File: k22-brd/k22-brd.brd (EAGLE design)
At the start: 22.9 x 63.5 mm, 34 parts, among them J1 61302011121, J2 61302011121, J3 CORTEX_DEBUG_PTH

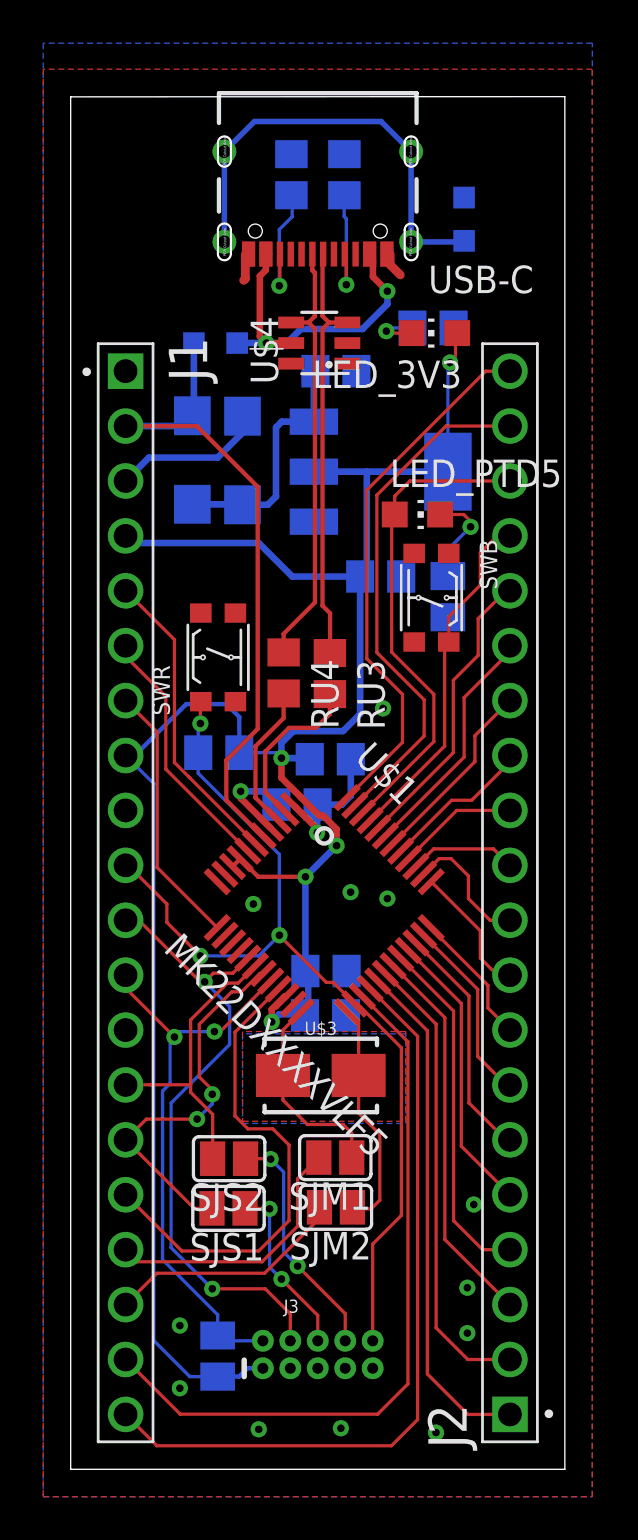
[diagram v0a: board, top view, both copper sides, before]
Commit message: prezehleno
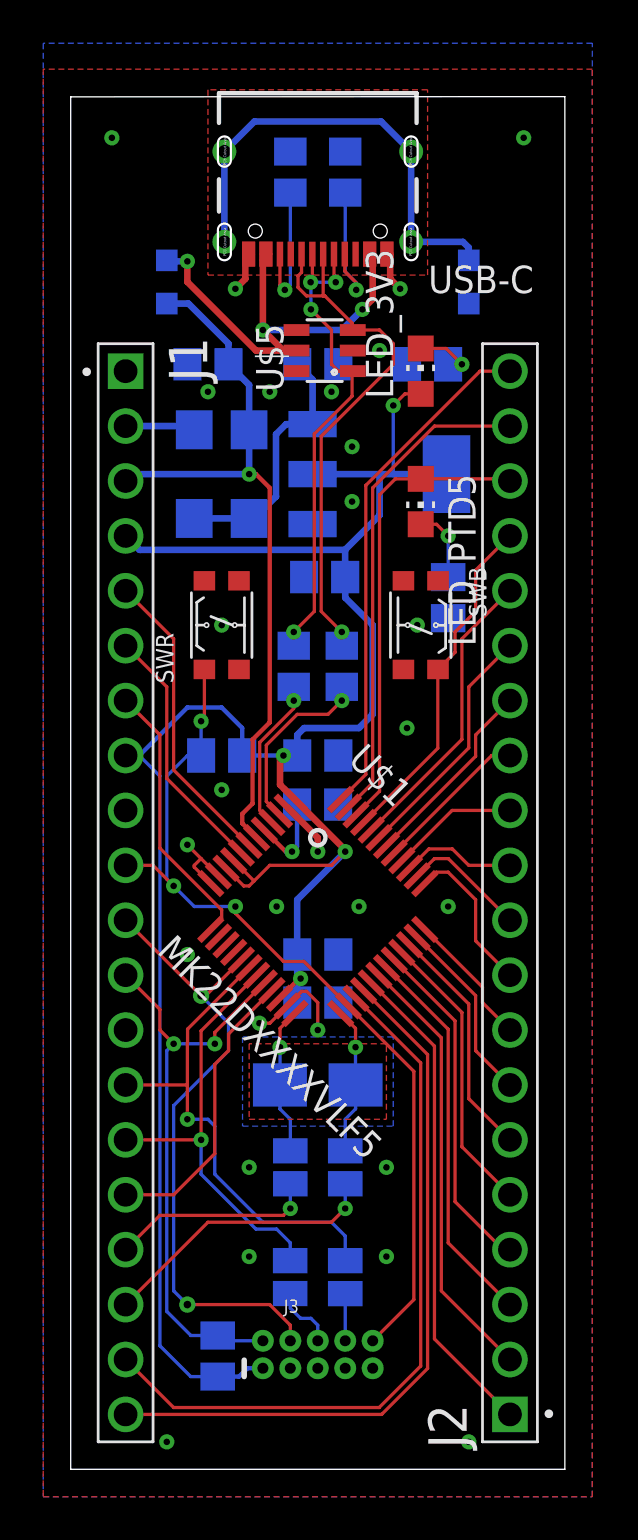
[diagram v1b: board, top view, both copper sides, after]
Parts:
- removed U$4: USBLC6-4SC6Y, vym0038_k22_misc:SOT23-6L
- added CU1: <1,10>u, rcl:C0805
- added U$5: USBLC6-2SC6, vym0038_k22_misc:SOT23-6L
- moved SJS2 7.67 mm to (12.7, 8.89), flipped to the bottom, turned to 90 degrees
- moved SJS1 4.27 mm to (10.2, 8.89), flipped to the bottom, turned to 90 degrees
- moved LU1 3.62 mm to (4.45, 54.9), turned to 90 degrees
- moved LU2 2.91 mm to (18.4, 54.9), turned to 90 degrees
- moved DV1 2.70 mm to (8.26, 46.0)
- moved CV2 2.59 mm to (11.7, 41.3), turned to 0 degrees
- moved DV2 2.32 mm to (5.71, 46.0)
- moved SJM1 2.13 mm to (10.2, 14.0), flipped to the bottom, turned to 270 degrees
- moved SJM2 1.90 mm to (12.7, 14.0), flipped to the bottom, turned to 270 degrees
- moved LED_3V3 1.87 mm to (16.2, 50.8), turned to 0 degrees
- moved RV1 1.70 mm to (16.5, 51.1), turned to 0 degrees
- moved SWR 1.50 mm to (6.99, 39.1)
- moved SWB 1.36 mm to (16.2, 39.1)
- moved CM4 0.95 mm to (11.4, 30.8)
- moved CV1 0.90 mm to (11.4, 51.1)
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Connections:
- net D+CON: now also U$5.3, U$5.4; no longer U$4.3
- net D-CON: now also U$5.1, U$5.6; no longer U$4.4
- net GND: now also CU1.1, U$5.2; no longer U$4.2
- net USB5V: now also CU1.2, J1.3; no longer J1.2
- net VBUSCON: now also U$5.5; no longer U$4.5
- net VIN: now also J1.2; no longer J1.3
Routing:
- net UART_RX: track 13.9 -> 23.0 mm, vias 0 -> 1
- net PTA4: track 22.5 -> 13.6 mm
- net N$3: track 11.0 -> 2.18 mm, vias 2 -> 0
- net GND: track 8.83 -> 15.3 mm, vias 13 -> 28
- net VBUSCON: track 16.6 -> 22.2 mm, vias 2 -> 3
- net N$4: track 8.17 -> 2.99 mm, vias 2 -> 0
- net D+CON: track 20.0 -> 24.9 mm, vias 0 -> 1
- net PTA19_OSC: track 10.8 -> 6.84 mm, vias 0 -> 1
- net VIN: track 7.10 -> 3.25 mm
- net PTA18: track 12.5 -> 9.55 mm, vias 0 -> 1
- net D-CON: track 20.1 -> 23.0 mm, vias 0 -> 4
- net PTA18_OSC: track 9.39 -> 6.84 mm, vias 0 -> 1
- net USB5V: track 31.6 -> 34.1 mm, vias 0 -> 1
- net UART_TX: track 17.9 -> 20.0 mm, vias 2 -> 1
- net RESET: track 44.1 -> 42.0 mm
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
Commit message: Nejake zmeny
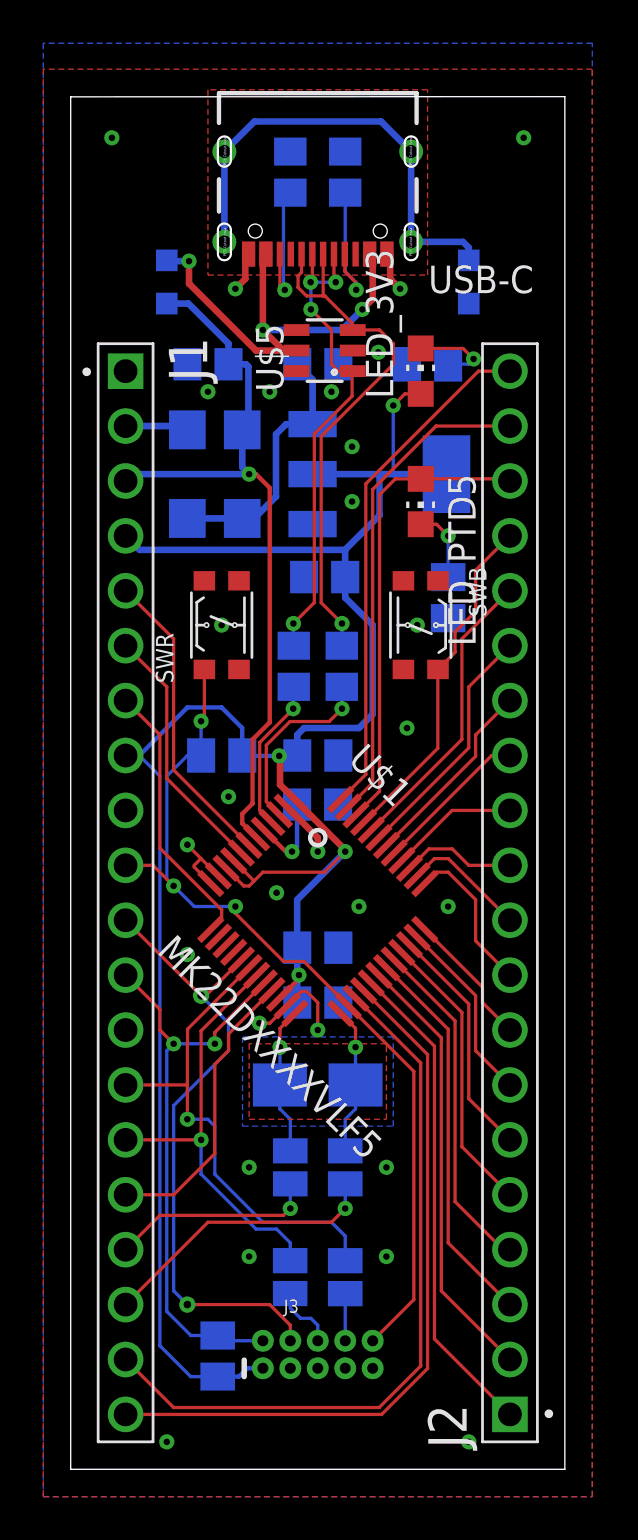
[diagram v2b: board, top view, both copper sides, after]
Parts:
- moved DV1 0.32 mm to (7.94, 46.0)
- moved DV2 0.32 mm to (5.40, 46.0)
- moved CM2 0.32 mm to (11.4, 24.1)
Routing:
- net N$2: track 2.85 -> 3.92 mm
- net USB5V: track 34.1 -> 34.8 mm
